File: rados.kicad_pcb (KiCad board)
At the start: 2 copper layers, 83.2 x 106 mm, 155 parts, among them J1 HEADER, J10 STEPSTICK, J11 STEPSTICK, J12 STEPSTICK, J13 MICROSD_SLOT_TFP09-2-12B, J2 HEADER, J3 HEADER, J4 STEPSTICK, J5 STEPSTICK, J6 STEPSTICK, J7 HEADER, J8 HEADER, J9 HEADER, P1 CONN_01X02, P10 CONN_01X04, P11 CONN_01X04, P12 CONN_01X04, P13 EXT_SD, P14 LCD, P15 LIMIT_SWITCHES, P16 LIMIT_SWITCHES_V, P17 CONN_01X03, P18 CONN_01X03, P19 CONN_01X03, P2 CONN_01X02, P20 CONN_01X03, P21 THERMISTORS, P22 CONN_01X05, P3 CONN_01X02, P4 CONN_01X02, P5 HP_MOSFETS, P6 MP_MOSFETS, P7 CONN_02X04, P8 CONN_01X04, P9 CONN_01X04, Q1 2N7002P, Q10 2N7002P, Q11 2N7002P, Q12 BC846BPDW1, Q13 BC846BPDW1, Q14 SI2318CDS-T1-GE3, Q15 IRFB7545PbF, Q16 2N7002P, Q17 2N7002P, Q18 BC846BPDW1, Q19 BC846BPDW1, Q2 2N7002P, Q20 SI2318CDS-T1-GE3, Q21 IRFB7545PbF, Q3 2N7002P, Q4 BC846BPDW1, Q5 BC846BPDW1, Q6 BC846BPDW1, Q7 IRFB7545PbF, Q8 SI2318CDS-T1-GE3, Q9 IRFB7545PbF, SW1 RESET, U1 MC34063, U2 24LC256

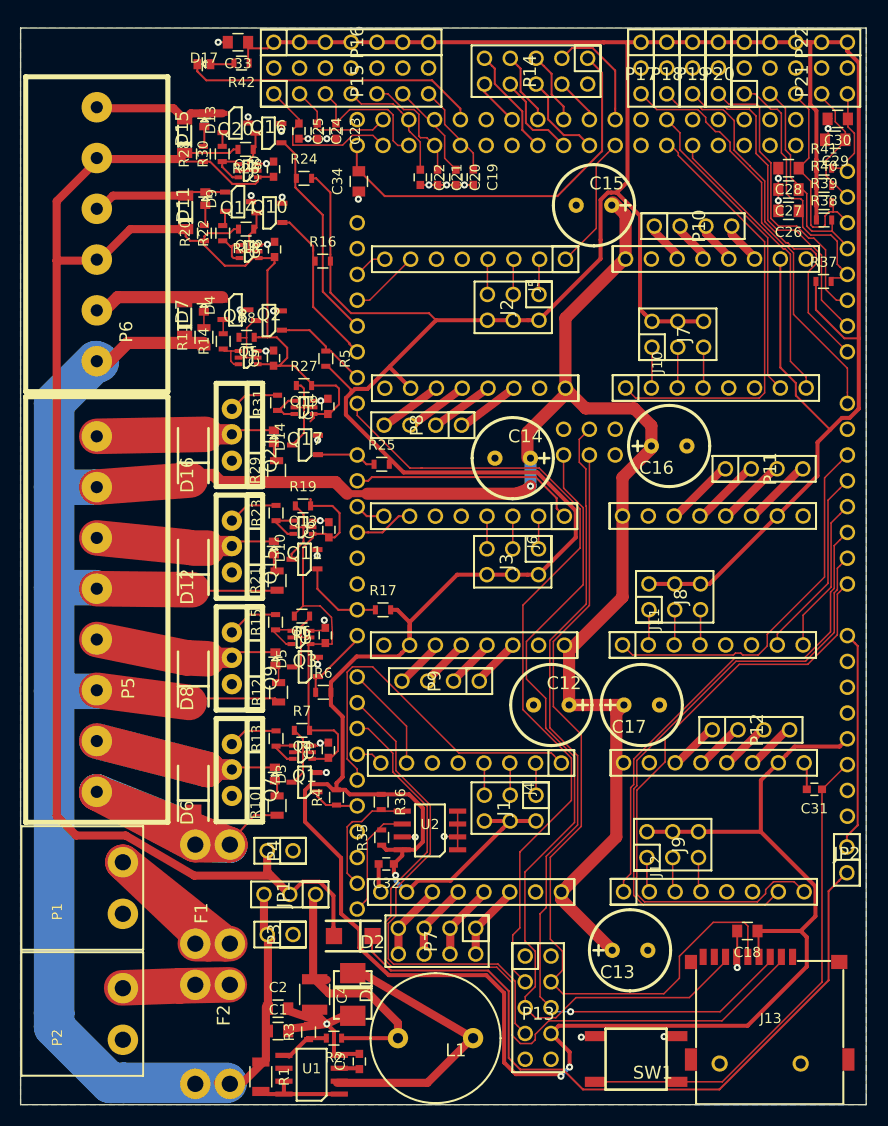
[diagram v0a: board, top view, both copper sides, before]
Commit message: cleanup
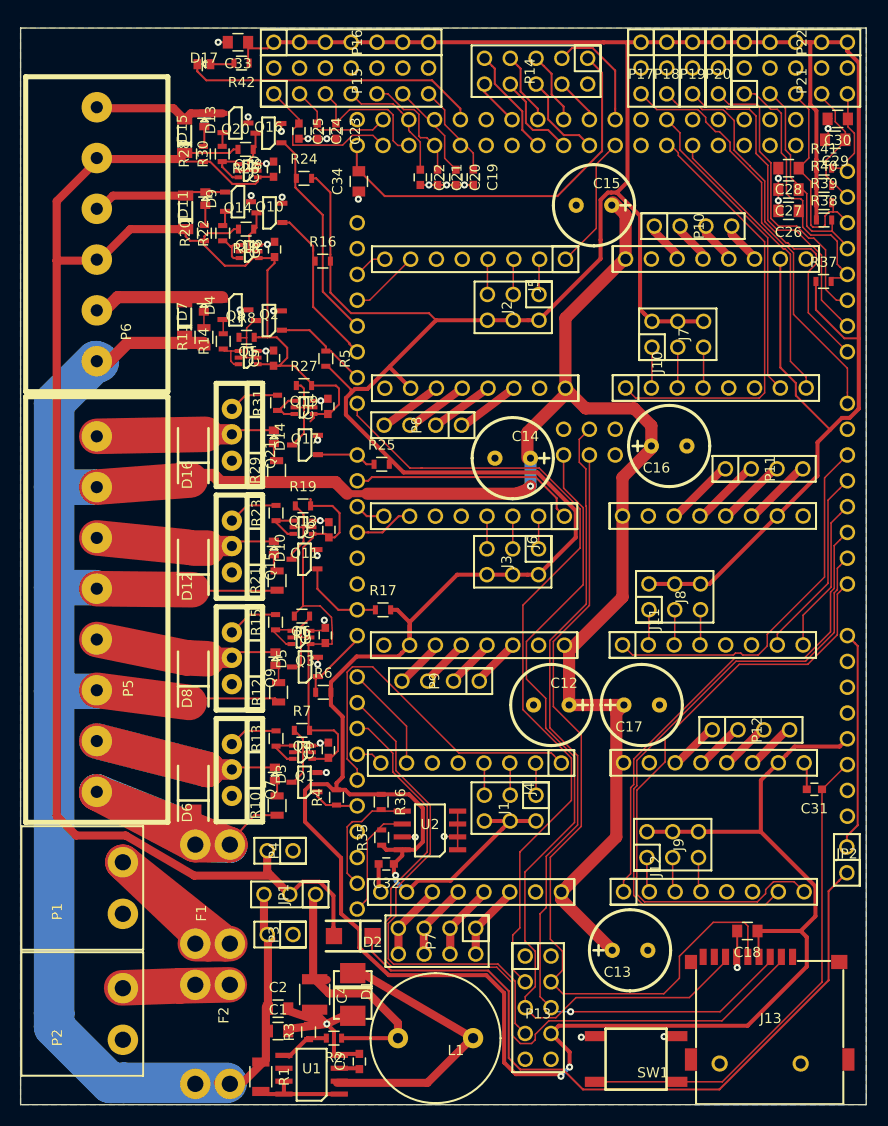
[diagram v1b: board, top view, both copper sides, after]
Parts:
- Q15, Q21, Q7, Q9: footprint to:TO-220 -> to:TO-220-3
